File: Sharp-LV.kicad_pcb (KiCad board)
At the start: 4 copper layers, 73.4 x 44.7 mm, 35 parts, among them J1 USB_C_Receptacle_USB2.0, J2 Conn_01x05_PROG, U1 NRF52840-QIAA-R, U2 USBLC6-2P6, U3 MCP1700-3302E_SOT23, U4 RT9080-33GJ5, Y1 32.768K, Y2 32.768K

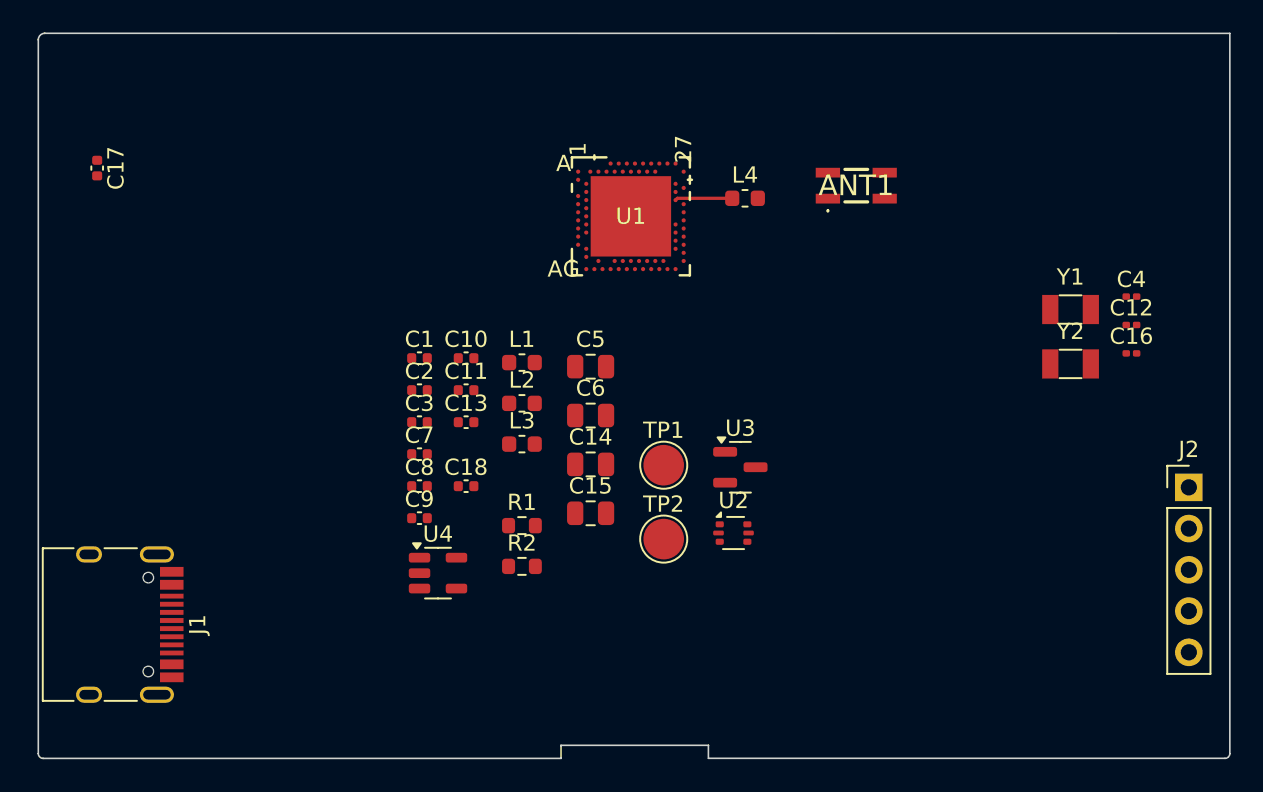
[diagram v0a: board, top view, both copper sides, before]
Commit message: Release 1.0 pending review
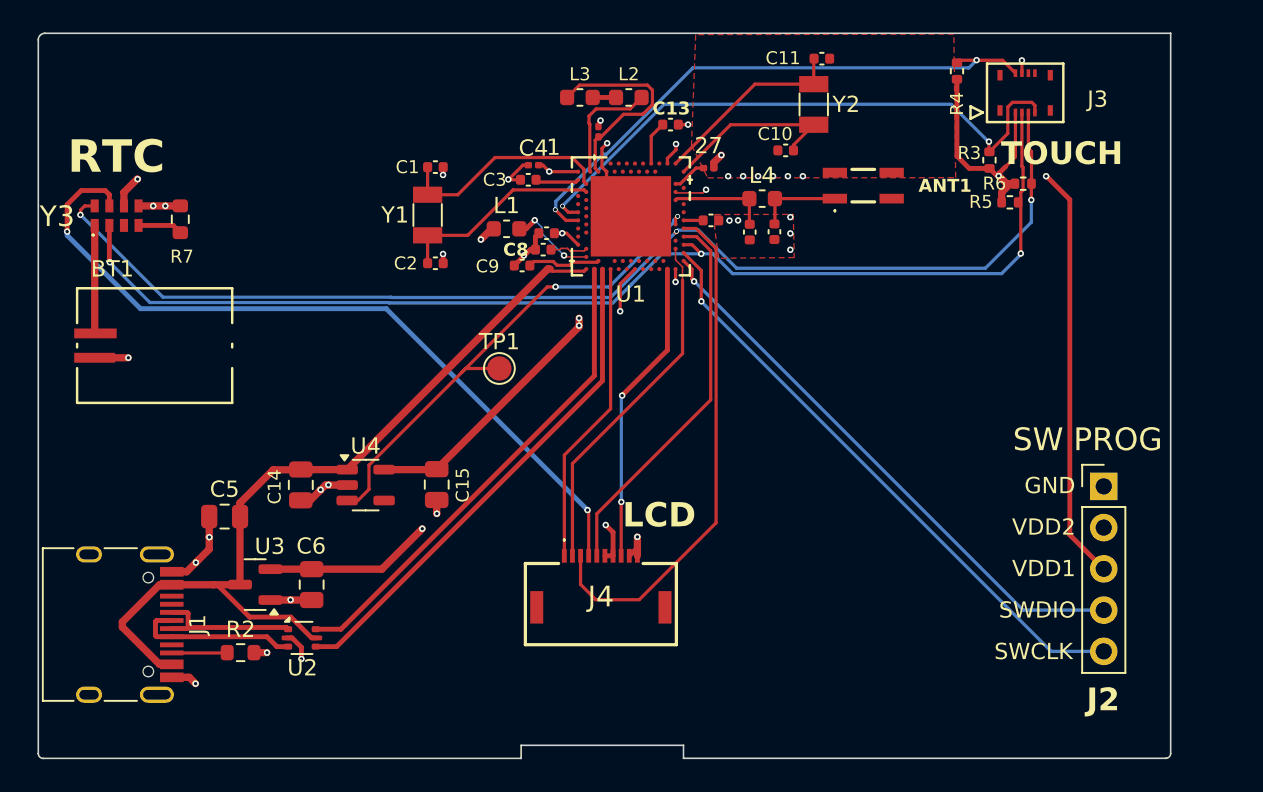
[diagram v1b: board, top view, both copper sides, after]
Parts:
- removed R1: 5.1k, Resistor_SMD:R_0603_1608Metric
- removed TP2: VDD1, TestPoint:TestPoint_Pad_D2.5mm
- added BT1: Battery_Cell, Footprints:CoinBattery_MS621FE, F.Cu at (106.4, 62.1)
- added C19: 820pF, Capacitor_SMD:C_0402_1005Metric, F.Cu at (140.7, 54.4)
- added J3: 5024260810, Footprints:CON_Molex_5024260812, F.Cu at (160.0, 46.6)
- added J4: FH52-10S-0.5SH_99, Footprints:FH5210S05SH99_LCD, F.Cu at (133.9, 78.1)
- added R3: 3.3k, Resistor_SMD:R_0402_1005Metric, F.Cu at (157.8, 50.7)
- added R4: 3.3k, Resistor_SMD:R_0402_1005Metric, F.Cu at (155.8, 45.2)
- added R5: 3.3k, Resistor_SMD:R_0402_1005Metric, F.Cu at (159.1, 53.3)
- added R6: 3.3k, Resistor_SMD:R_0402_1005Metric, F.Cu at (159.9, 52.2)
- added R7: 5.1k, Resistor_SMD:R_0603_1608Metric, F.Cu at (108.0, 54.4)
- added Y3: RV-3032-C7, Footprints:RV3032C7, F.Cu at (104.1, 54.1)
- C10, C11: value 22pF -> 12pF
- TP1: footprint TestPoint:TestPoint_Pad_D2.5mm -> TestPoint:TestPoint_Pad_D1.5mm
- moved C17 41.9 mm to (144.6, 55.1), turned to 90 degrees
- moved Y1 40.0 mm to (123.2, 54.1), turned to 90 degrees
- moved C4 37.7 mm to (129.8, 51.0)
- moved C16 35.6 mm to (133.8, 49.0), turned to -90 degrees
- moved U3 30.7 mm to (112.6, 76.9), turned to 180 degrees
- moved C11 29.9 mm to (147.5, 44.5), turned to 180 degrees
- moved C12 27.8 mm to (140.6, 51.2), turned to 180 degrees
- moved U2 27.4 mm to (115.5, 80.2)
- moved C5 24.4 mm to (110.7, 72.7)
- moved C10 23.5 mm to (145.3, 50.1)
- moved C18 23.5 mm to (143.1, 55.2), turned to 90 degrees
- moved Y2 22.5 mm to (147.0, 47.3), turned to -90 degrees
- moved C13 22.2 mm to (138.2, 48.5), turned to 180 degrees
- moved L3 21.6 mm to (132.6, 46.9)
- moved C6 20.1 mm to (116.1, 76.9), turned to 90 degrees
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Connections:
- C14 pad 1: VIN -> VBUS
- J1 pad A5: Net-(J1-CC1) -> unconnected-(J1-CC1-PadA5)
- J1 pad A6: /USB_D+ -> /USB_IN_D+
- J1 pad A7: /USB_D- -> /USB_IN_D-
- J1 pad B6: /USB_D+ -> /USB_IN_D+
- J1 pad B7: /USB_D- -> /USB_IN_D-
- J2 pad 3: /RESET -> VDD
- U1 pad AC13: /RESET -> unconnected-(U1-P0.18/NRESET-PadAC13)
- U1 pad AD22: unconnected-(U1-P1.00-PadAD22) -> /LCD_EXTMODE
- U1 pad AD8: unconnected-(U1-P0.13-PadAD8) -> /SPI_CLK
- U1 pad L1: unconnected-(U1-P0.06-PadL1) -> /TOUCH_REST
- U1 pad N1: unconnected-(U1-P0.08-PadN1) -> /TOUCH_IRQ
- U1 pad N24: unconnected-(U1-DEC5-PadN24) -> Net-(U1-DEC5)
- U1 pad P2: unconnected-(U1-P1.08-PadP2) -> /SPI_MISO
- U1 pad R24: unconnected-(U1-P1.06-PadR24) -> /LCD_CS
- U1 pad U24: unconnected-(U1-P1.04-PadU24) -> /LCD_DISPON
- U1 pad Y23: unconnected-(U1-P1.01-PadY23) -> /SPI_MOSI
- U2 pad 1: /USB_U_D- -> /USB_IN_D-
- U2 pad 3: /USB_U_D+ -> /USB_IN_D+
- U4 pad 1: VIN -> VBUS
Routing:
- net VDD: track 0.00 -> 152.2 mm, vias 0 -> 7
- net VDD2: track 0.00 -> 84.5 mm, vias 0 -> 6
- net /SCL: track 0.00 -> 72.8 mm, vias 0 -> 3
- net /SDA: track 0.00 -> 72.0 mm, vias 0 -> 3
- net VBUS: track 0.00 -> 52.1 mm
- net /RTC_SQW: track 0.00 -> 47.4 mm, vias 0 -> 2
- net /SWCLK: track 0.00 -> 37.2 mm, vias 0 -> 1
- net /TOUCH_REST: track 0.00 -> 37.1 mm, vias 0 -> 2
- net GND: track 0.00 -> 36.8 mm, vias 0 -> 34
- net /TOUCH_IRQ: track 0.00 -> 35.7 mm, vias 0 -> 2
- net /SWDIO: track 0.00 -> 35.1 mm, vias 0 -> 1
- net /LCD_CS: track 0.00 -> 31.9 mm
- net /VDD2_ENABLE: track 0.00 -> 31.5 mm, vias 0 -> 2
- net /USB_D+: track 0.00 -> 31.3 mm
- net /USB_D-: track 0.00 -> 30.2 mm
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- added copper zone on F.Cu, net GND
- added copper zone on In1.Cu, net GND
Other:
- board size 73.4 x 44.7 mm -> 69.7 x 44.7 mm
- board text added: "GND"
- board text added: "LCD"
- board text added: "RTC"
- board text added: "SW PROG"
- board text added: "SWCLK"
- board text added: "SWDIO"
- board text added: "TOUCH"
- board text added: "VDD1"
- board text added: "VDD2"
